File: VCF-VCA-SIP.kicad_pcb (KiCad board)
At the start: 2 copper layers, 40 x 18 mm, 44 parts, among them P1 CONN_10, Q1 BC857BS, U1 LM13700, U2 TL074-, U3 LM13700, U4 LM13700, U5 TL072-

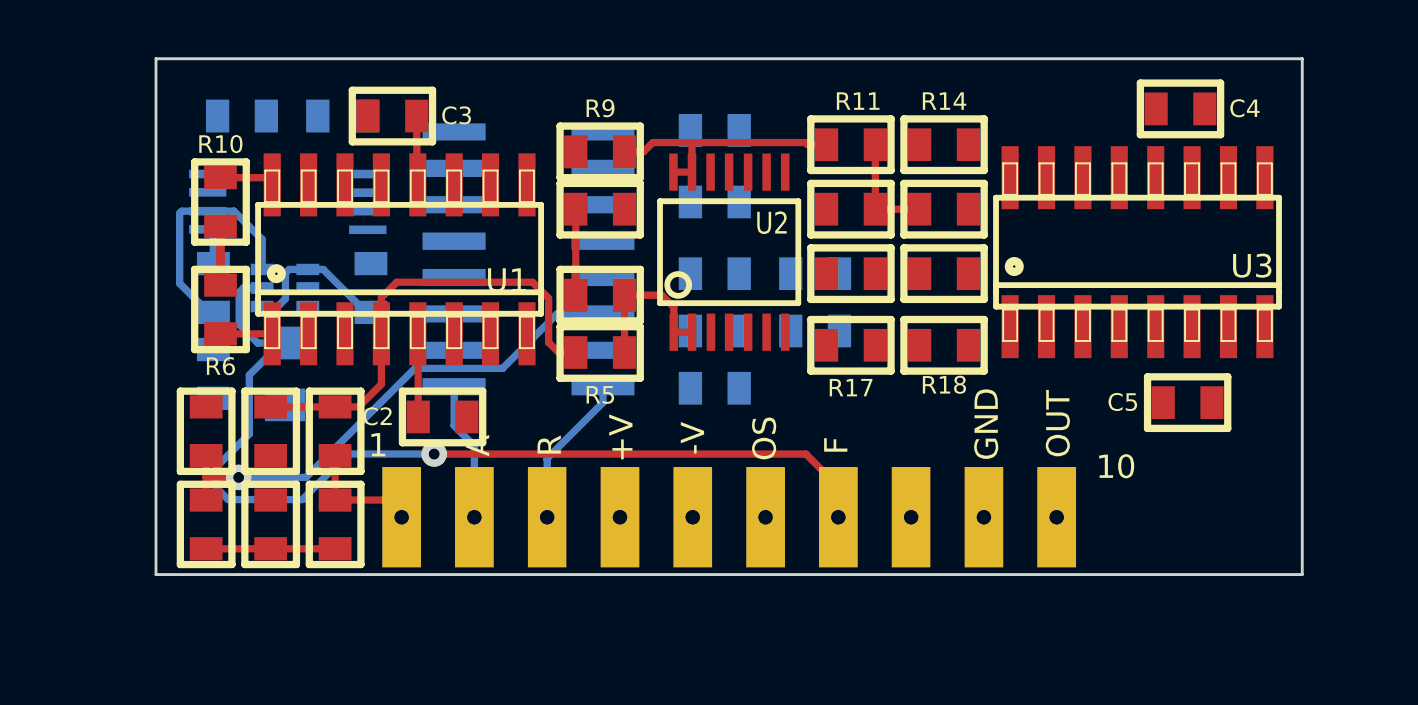
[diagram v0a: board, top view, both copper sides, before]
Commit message: routing
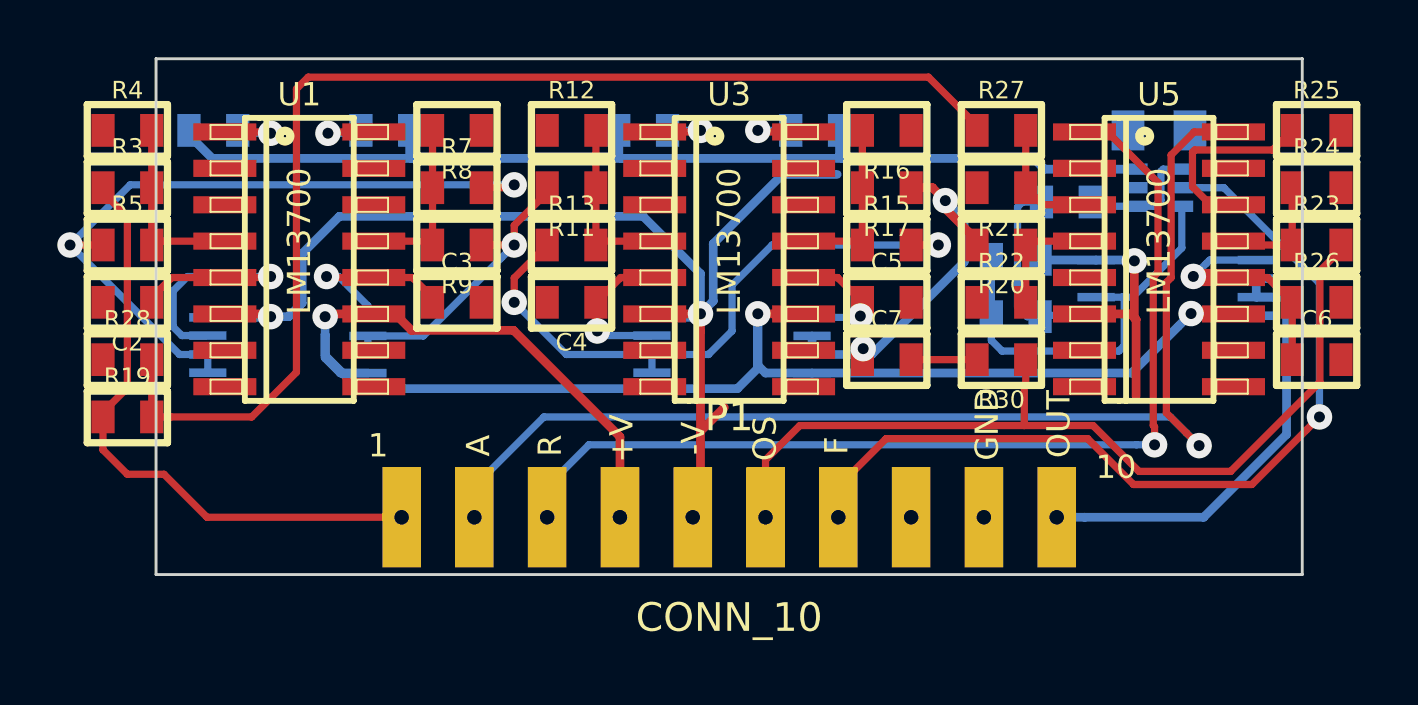
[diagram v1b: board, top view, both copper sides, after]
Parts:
- added U6: TL072-, MyModules:TSSOP8-JRL, B.Cu at (133.5, 91.0)
- C1, C2, C3, C4, C5: footprint SM0603-JRL -> MyModules:SM0603-C-JRL
- C6: footprint SM0603-JRL -> MyModules:SM0603-C-JRL; moved to F.Cu
- C7: footprint synth:SM0603-JRL -> MyModules:SM0603-C-JRL; moved to F.Cu
- P1: footprint CONN_10X_0100_SMD_THRUHOLE -> synth:CONN_10X_0100_SMD_THRUHOLE
- Q1: footprint SOT363-JRL -> MyModules:SOT363-JRL
- R1, R11, R12, R13, R15, R16, R17, R19, R2, R21, R27, R28, R3, R4, R5, R7, R8, R9: footprint SM0603-JRL -> MyModules:SM0603-R-JRL
- R10, R14, R18, R6: footprint SM0603-JRL -> MyModules:SM0603-R-JRL; moved to B.Cu
- R20, R22, R23, R24, R25, R26, R30: footprint SM0603-JRL -> MyModules:SM0603-R-JRL; moved to F.Cu
- R29: footprint SM0805-HAND -> MyModules:SM0805-HAND
- U1, U3: footprint SO16-JRL -> MyModules:SO16-JRL
- U2: value TL074- -> TL072-; footprint TSSOP14 -> MyModules:TSSOP8-JRL; moved to B.Cu
- U4: value LM13700 -> TL072-; footprint SO16-JRL -> MyModules:TSSOP8-JRL
- U5: value TL072- -> LM13700; footprint TSSOP8-JRL -> MyModules:SO16-JRL; moved to F.Cu
- moved C6 38.5 mm to (138.5, 93.5), turned to 0 degrees
- moved R26 34.6 mm to (138.5, 91.5)
- moved R29 31.7 mm to (133.0, 85.5), turned to 180 degrees
- moved R27 31.0 mm to (127.5, 85.5), turned to 0 degrees
- moved Q1 30.7 mm to (133.0, 87.5), turned to 90 degrees
- moved U5 30.6 mm to (133.0, 90.0), turned to 270 degrees
- moved R21 29.0 mm to (127.5, 87.5), turned to 180 degrees
- moved R1 28.3 mm to (128.0, 90.0), turned to 0 degrees
- moved C1 28.0 mm to (128.0, 92.0), turned to 180 degrees
- moved R2 24.4 mm to (129.8, 88.0), turned to 180 degrees
- moved R25 22.8 mm to (138.5, 85.5)
- moved C4 22.3 mm to (112.5, 91.5), turned to 180 degrees
- moved R23 21.2 mm to (138.5, 89.5)
- moved R24 21.2 mm to (138.5, 87.5)
- moved R5 16.9 mm to (97.0, 89.5), turned to 0 degrees
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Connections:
- U2 pad 4: +VCC -> -VCC
- U2 pad 5: Net-(C5-Pad1) -> Net-(C3-Pad1)
- U2 pad 6: VCF_OUT -> Net-(R11-Pad2)
- U2 pad 7: VCF_OUT -> Net-(R11-Pad2)
- U2 pad 8: Net-(R13-Pad1) -> +VCC
- U3 pad 1: Net-(R18-Pad1) -> Net-(R14-Pad1)
- U3 pad 12: Net-(C4-Pad1) -> Net-(C5-Pad1)
- U3 pad 13: Net-(R11-Pad1) -> Net-(R15-Pad1)
- U3 pad 16: Net-(R14-Pad1) -> Net-(R18-Pad1)
- U3 pad 4: Net-(R15-Pad1) -> Net-(R11-Pad1)
- U3 pad 5: Net-(C5-Pad1) -> Net-(C4-Pad1)
- U4 pad 1: VCA_CTRL -> Net-(R13-Pad1)
- U4 pad 2: Net-(U4-Pad2) -> Net-(R13-Pad1)
- U4 pad 3: Net-(R25-Pad1) -> Net-(C4-Pad1)
- U4 pad 4: Net-(R23-Pad1) -> -VCC
- U4 pad 5: Net-(C6-Pad1) -> Net-(C5-Pad1)
- U4 pad 6: -VCC -> VCF_OUT
- U4 pad 7: (no net) -> VCF_OUT
- U4 pad 8: (no net) -> +VCC
- U5 pad 1: Net-(C1-Pad1) -> RES_CTRL
- U5 pad 2: Net-(C1-Pad2) -> Net-(U5-Pad2)
- U5 pad 3: GND -> Net-(R21-Pad1)
- U5 pad 4: -VCC -> Net-(R20-Pad1)
- U5 pad 5: Net-(C6-Pad1) -> Net-(R3-Pad2)
- U5 pad 6: VCA_OUT -> -VCC
- U5 pad 7: VCA_OUT -> (no net)
- U5 pad 8: +VCC -> (no net)
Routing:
- net +VCC: track 0.00 -> 59.8 mm, vias 0 -> 3
- net -VCC: track 0.00 -> 53.4 mm, vias 0 -> 3
- net Net-(R19-Pad2): track 4.50 -> 42.4 mm
- net VCA_CTRL: track 4.85 -> 41.0 mm, vias 0 -> 1
- net Iabc: track 2.05 -> 36.8 mm
- net OFFSET: track 0.00 -> 31.2 mm
- net RES_CTRL: track 5.36 -> 35.4 mm, vias 0 -> 1
- net Net-(R13-Pad1): track 0.00 -> 22.1 mm, vias 0 -> 2
- net Net-(R5-Pad1): track 5.40 -> 25.7 mm, vias 0 -> 2
- net VCF_IN: track 4.12 -> 21.2 mm
- net VCA_OUT: track 0.00 -> 15.7 mm
- net VCF_OUT: track 0.00 -> 13.7 mm, vias 0 -> 2
- net Net-(R21-Pad1): track 17.8 -> 4.30 mm, vias 1 -> 0
- net Net-(R3-Pad2): track 16.1 -> 6.61 mm
- net Net-(C6-Pad1): track 0.00 -> 8.26 mm, vias 0 -> 1
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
